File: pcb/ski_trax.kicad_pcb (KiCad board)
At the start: 2 copper layers, 62.2 x 100.3 mm, 13 parts, among them SW1 SW_Push, SW2 SW_Push, SW3 SW_Push

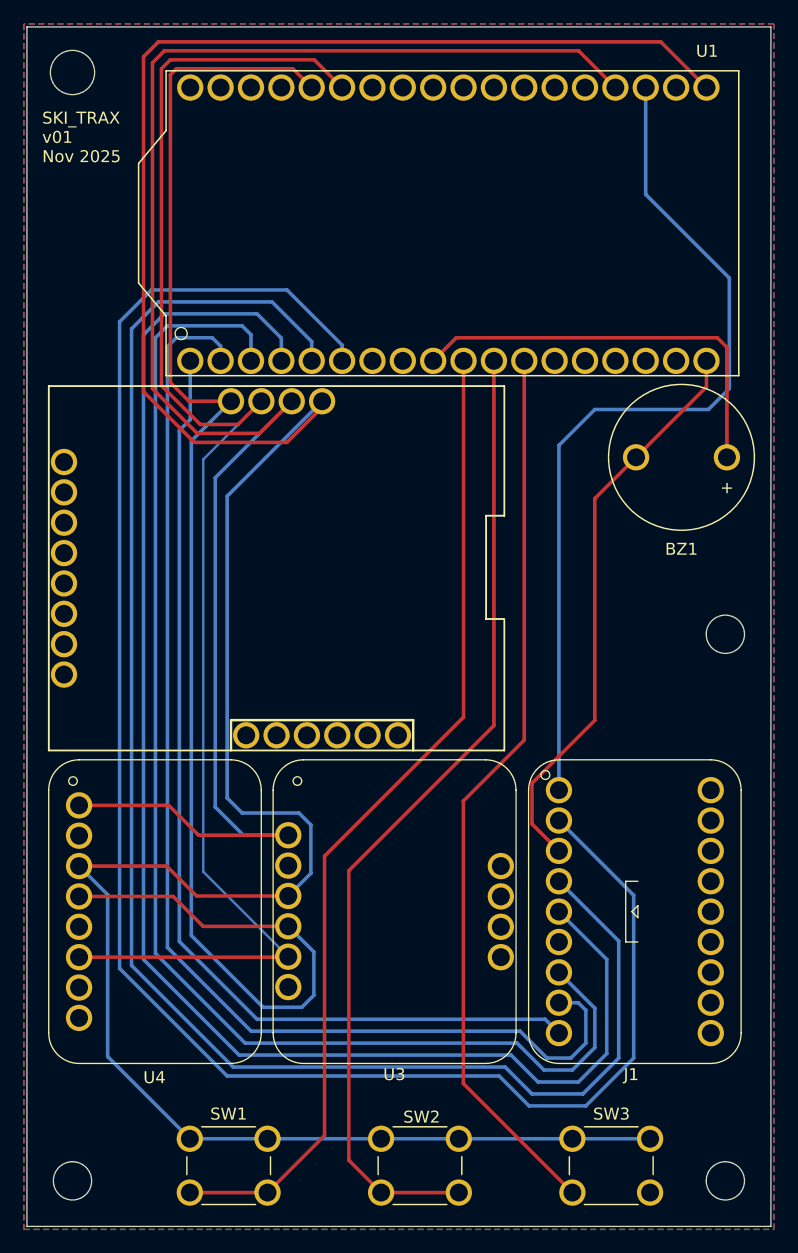
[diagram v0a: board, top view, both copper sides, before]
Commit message: Update PCB files
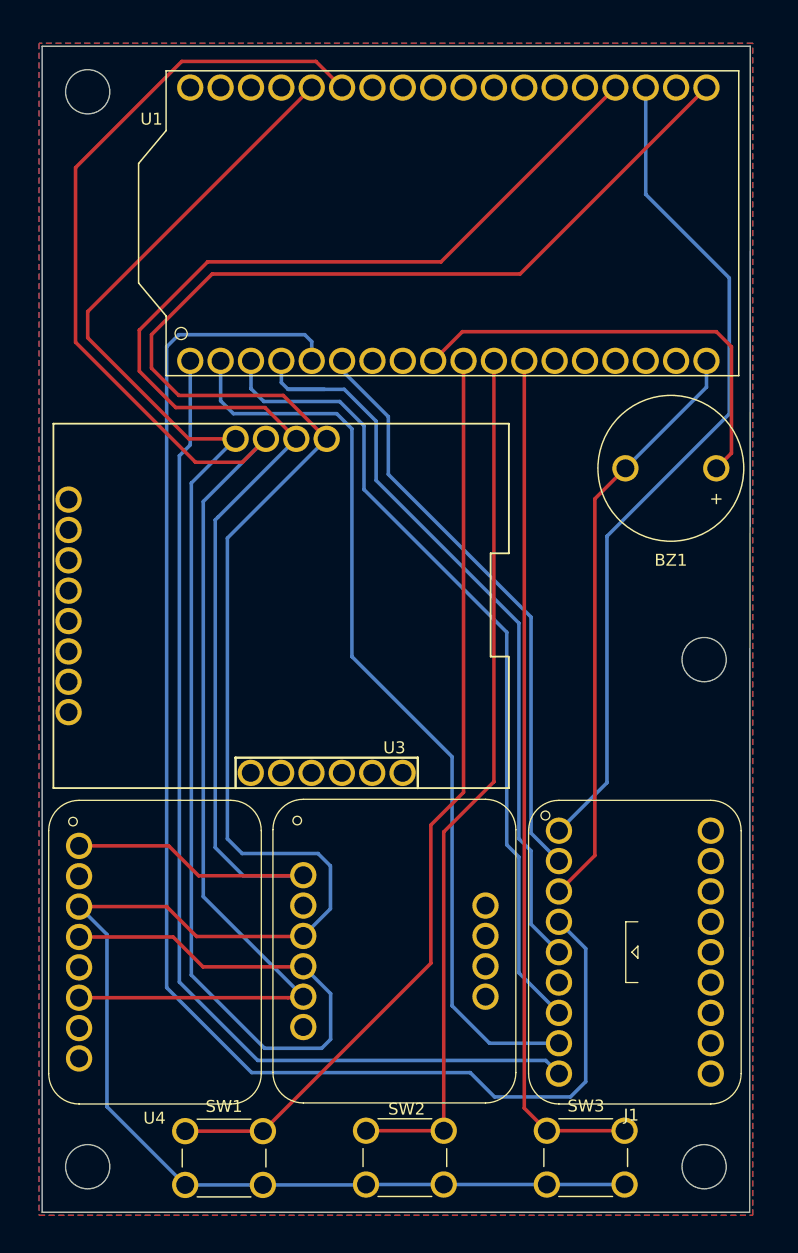
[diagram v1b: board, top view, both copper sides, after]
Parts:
- removed the REF** at (79.5, 74.1)
- removed the REF** at (79.5, 119.8)
- removed the REF** at (24.9, 119.8)
- added REF**: MountingHole_3.7mm, MountingHole:MountingHole_3.7mm, F.Cu at (77.7, 118.4)
- added REF**: MountingHole_3.7mm, MountingHole:MountingHole_3.7mm, F.Cu at (26.4, 118.6)
- added REF**: MountingHole_3.7mm, MountingHole:MountingHole_3.7mm, F.Cu at (78.0, 76.2)
- moved J1 3.39 mm to (71.7, 100.7)
- moved U4 3.39 mm to (31.8, 100.7)
- moved U3 3.30 mm to (51.8, 100.6)
- moved U2 3.17 mm to (23.2, 56.4)
- moved SW3 2.24 mm to (71.1, 120.1)
- moved REF** 2.05 mm to (26.2, 28.7)
- moved SW2 1.43 mm to (55.9, 120.1)
- moved BZ1 1.28 mm to (78.7, 60.2)
- moved SW1 0.75 mm to (40.8, 120.1)
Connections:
- SW1 pad 1: SW1 -> GND
- SW1 pad 2: GND -> SW1
- SW2 pad 1: SW2 -> GND
- SW2 pad 2: GND -> SW2
- SW3 pad 1: SW3 -> GND
- SW3 pad 2: GND -> SW3
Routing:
- net TFT_LITE: track 148.9 -> 49.4 mm
- net TFT_MOSI: track 124.8 -> 64.9 mm
- net TFT_DC: track 111.5 -> 69.5 mm
- net TFT_RST: track 101.3 -> 77.4 mm
- net GND: track 278.4 -> 261.2 mm
- net TFT_CLK: track 135.5 -> 121.7 mm
- net 3V3_1: track 144.2 -> 132.3 mm
- net SDA: track 122.3 -> 133.6 mm
- net SW2: track 82.2 -> 72.6 mm
- net SW1: track 82.9 -> 77.9 mm
- net SW3: track 75.5 -> 71.7 mm
- net SCL: track 128.5 -> 132.3 mm
- net TFT_LCDCS: track 83.9 -> 87.3 mm
- net BUZ: track 34.9 -> 37.2 mm
- net 3V3_2: track 73.6 -> 71.5 mm
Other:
- board size 62.2 x 100.3 mm -> 59.2 x 97.5 mm
- board text added: "SKI_TRAX v02 Nov 2025"
- board text removed: "SKI_TRAX v01 Nov 2025"
